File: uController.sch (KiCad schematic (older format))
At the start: 14 parts

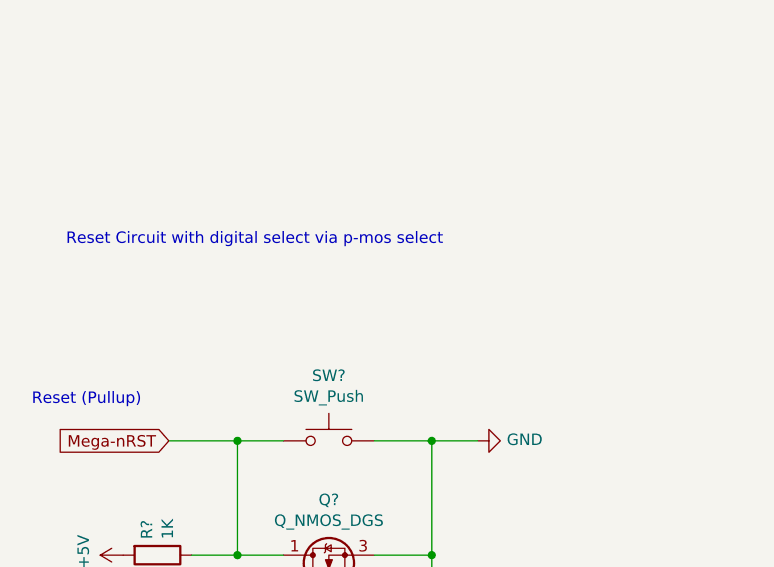
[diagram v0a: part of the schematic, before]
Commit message: updates
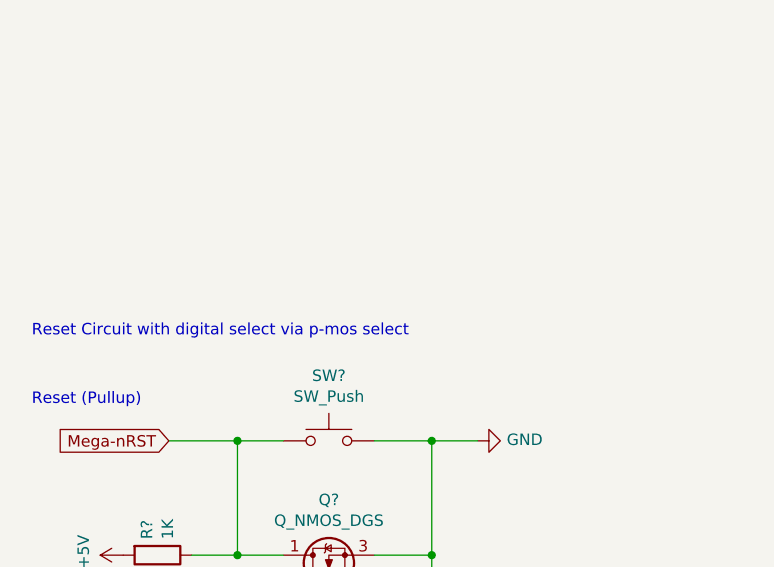
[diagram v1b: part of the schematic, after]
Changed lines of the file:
@@
 Wire Wire Line
 	1600 7100 1800 7100
-Text Notes 850  5750 0    50   ~ 0
+Text Notes 700  6150 0    50   ~ 0
 Reset Circuit with digital select via p-mos select\n
 Wire Wire Line

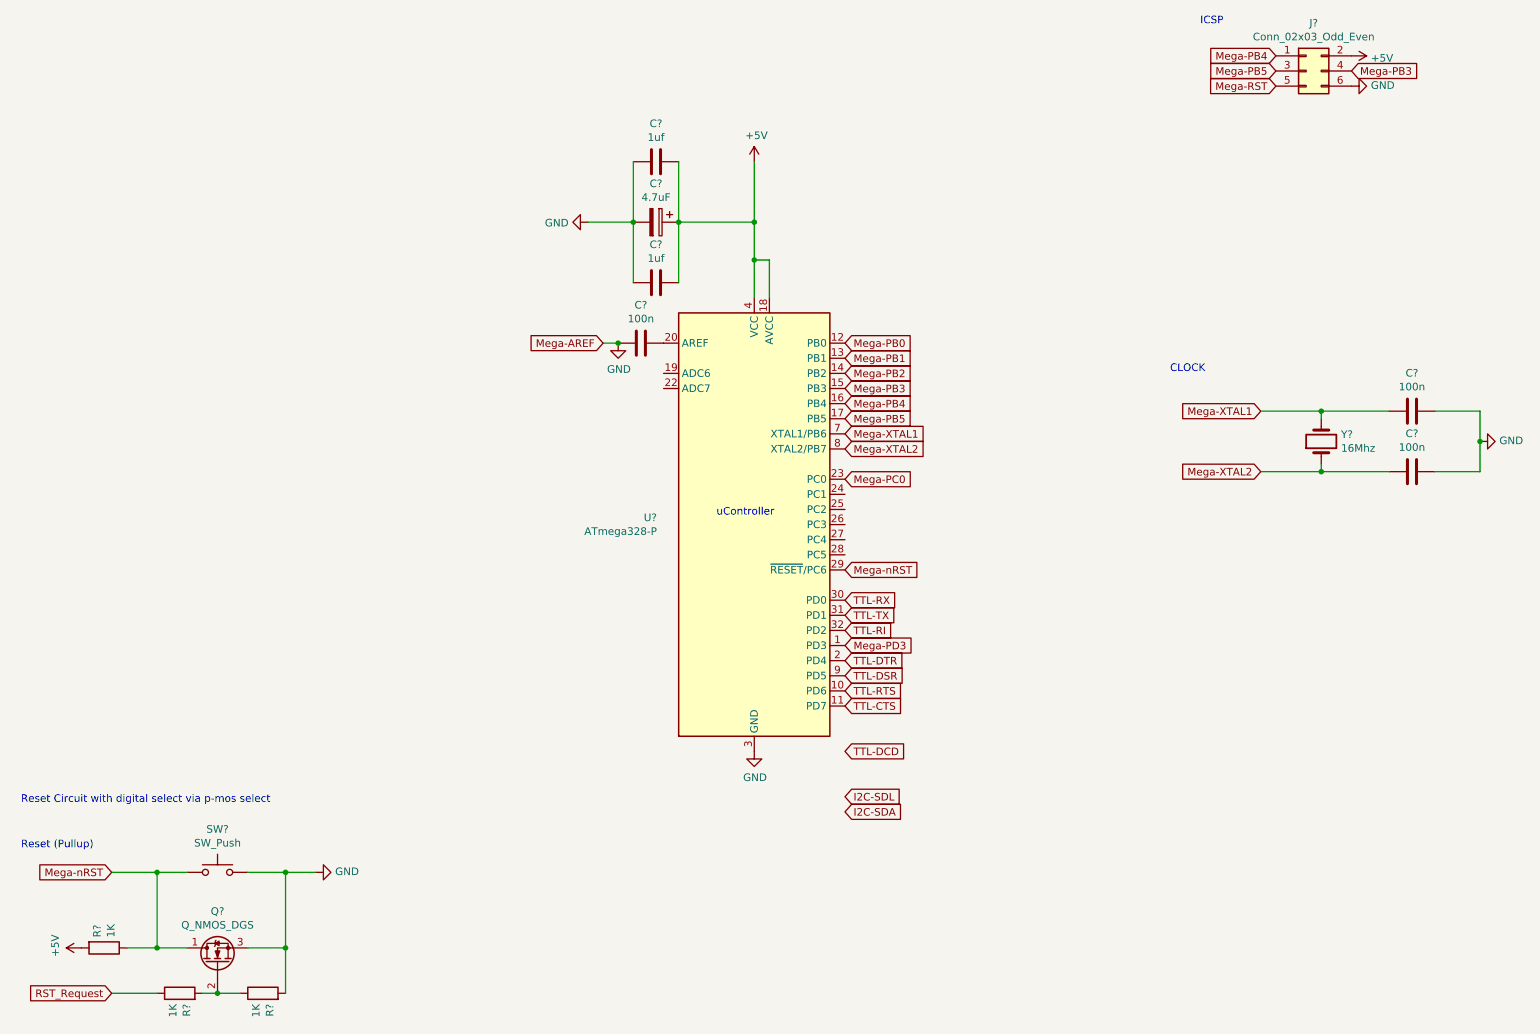
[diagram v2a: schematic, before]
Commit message: updates
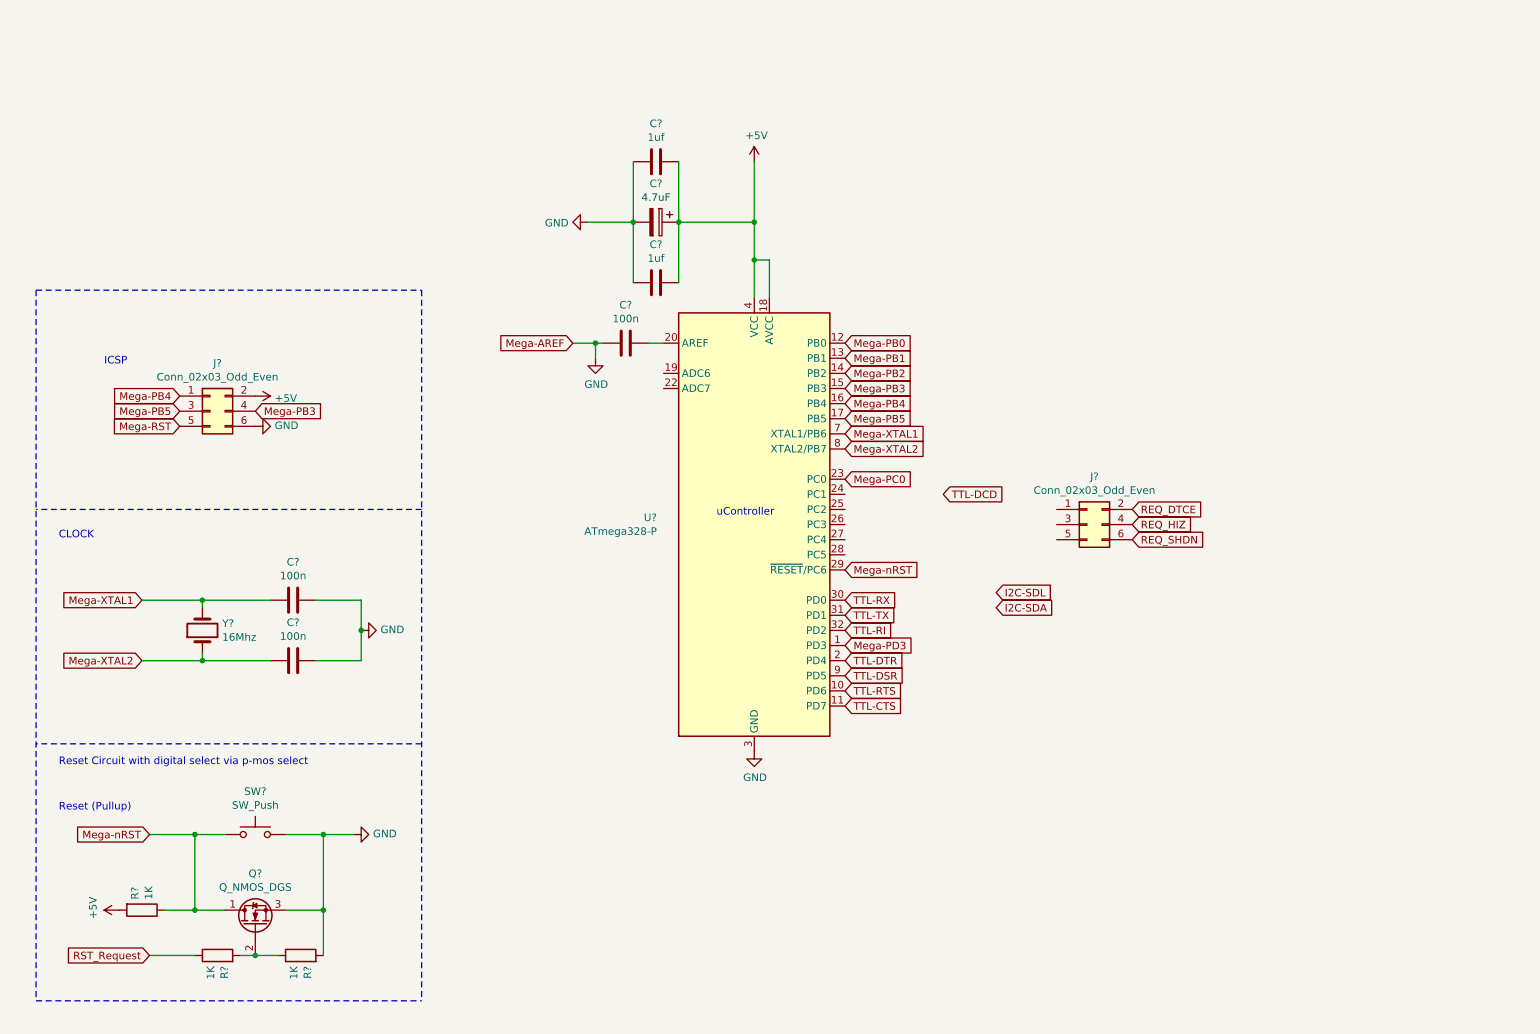
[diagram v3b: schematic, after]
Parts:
- added J?: Conn_02x03_Odd_Even, symbol Connector_Generic:Conn_02x03_Odd_Even
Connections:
- new net REQ_DTCE: J?.2 (Pin_2)
- new net REQ_HIZ: J?.4 (Pin_4)
- new net REQ_SHDN: J?.6 (Pin_6)
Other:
- moved on the sheet: C?, J?, Q?, R?, SW?, Y?
